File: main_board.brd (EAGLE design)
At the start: 91 x 66 mm, 49 parts, among them IC1 LT1168ACS8, IC2 LT1168ACS8, IC3 LT1168ACS8, IC4 317EMP, U1 TLC272IP, U2 TLC272IP, U3 TLC272IP

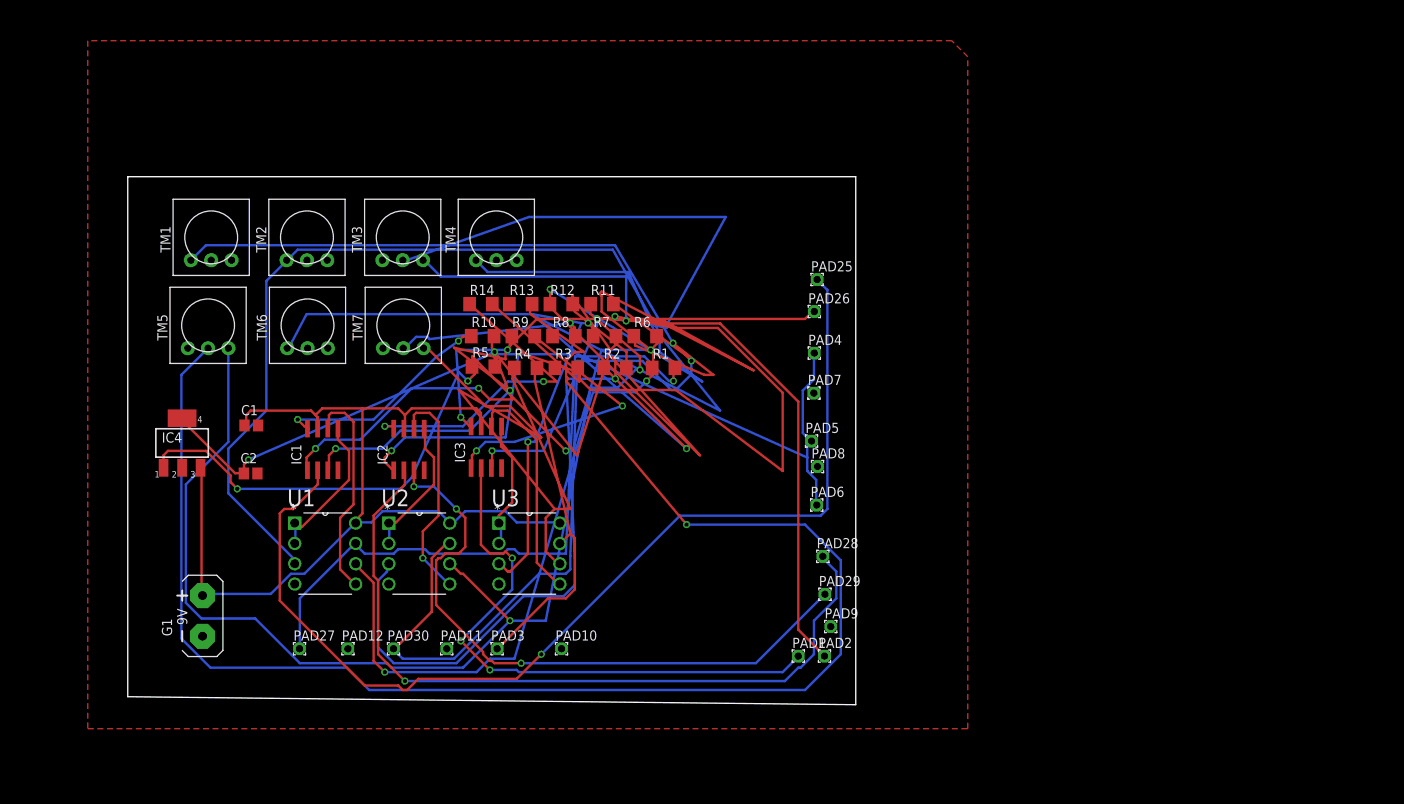
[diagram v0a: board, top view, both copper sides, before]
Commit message: Re-doing main board. Use this
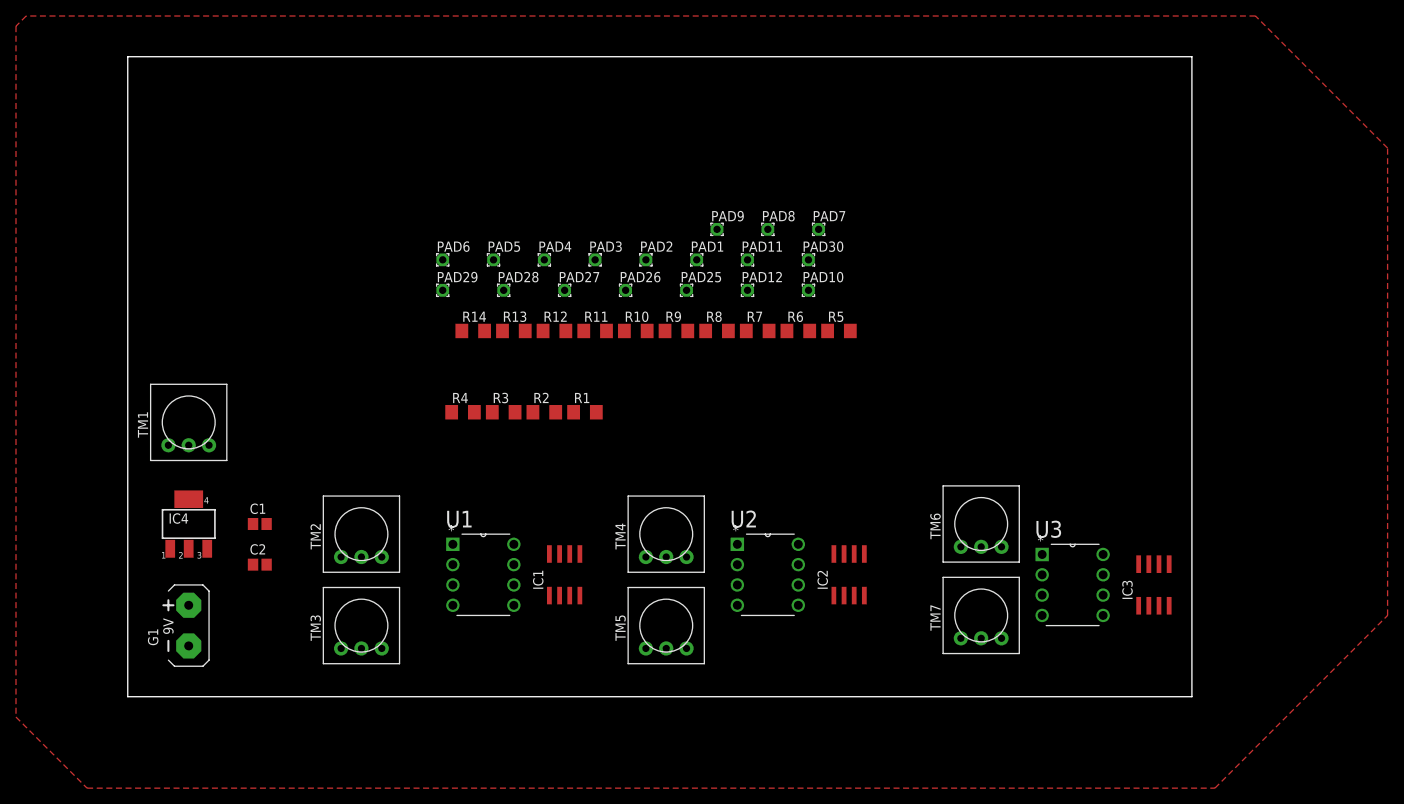
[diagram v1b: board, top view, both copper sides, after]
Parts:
- moved TM6 87.8 mm to (106.7, 21.6)
- moved IC3 85.2 mm to (128.3, 14.0)
- moved TM7 80.8 mm to (106.7, 10.2)
- moved PAD30 71.1 mm to (85.1, 54.6)
- moved TM5 68.5 mm to (67.3, 8.89)
- moved U3 68.0 mm to (121.9, 10.2)
- moved PAD12 67.1 mm to (77.5, 50.8)
- moved PAD11 61.5 mm to (77.5, 54.6)
- moved PAD29 61.0 mm to (39.4, 50.8)
- moved IC2 57.2 mm to (90.2, 15.2)
- moved PAD6 55.9 mm to (39.4, 54.6)
- moved PAD27 55.7 mm to (54.6, 50.8)
- moved PAD10 54.4 mm to (85.1, 50.8)
- moved PAD2 54.3 mm to (64.8, 54.6)
- moved PAD28 51.9 mm to (47.0, 50.8)
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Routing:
- net N$27: track 196.0 -> 0.00 mm, vias 1 -> 0
- net N$25: track 180.2 -> 0.00 mm, vias 2 -> 0
- net N$3: track 175.7 -> 0.00 mm, vias 1 -> 0
- net VDD: track 164.7 -> 0.00 mm, vias 2 -> 0
- net N$2: track 159.7 -> 0.00 mm, vias 3 -> 0
- net N$24: track 143.0 -> 0.00 mm, vias 2 -> 0
- net N$22: track 130.6 -> 0.00 mm, vias 1 -> 0
- net N$5: track 128.8 -> 0.00 mm, vias 1 -> 0
- net VCC: track 120.0 -> 0.00 mm
- net N$23: track 100.3 -> 0.00 mm, vias 1 -> 0
- net N$32: track 96.3 -> 0.00 mm, vias 1 -> 0
- net N$6: track 94.3 -> 0.00 mm, vias 4 -> 0
- net N$17: track 89.1 -> 0.00 mm, vias 2 -> 0
- net N$10: track 86.3 -> 0.00 mm, vias 1 -> 0
- net N$21: track 85.3 -> 0.00 mm, vias 2 -> 0
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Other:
- board size 91 x 66 mm -> 133 x 80 mm
